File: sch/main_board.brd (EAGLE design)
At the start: 99.2 x 65.2 mm, 17 parts, among them IC1 MCP73831T-2ACI_OT

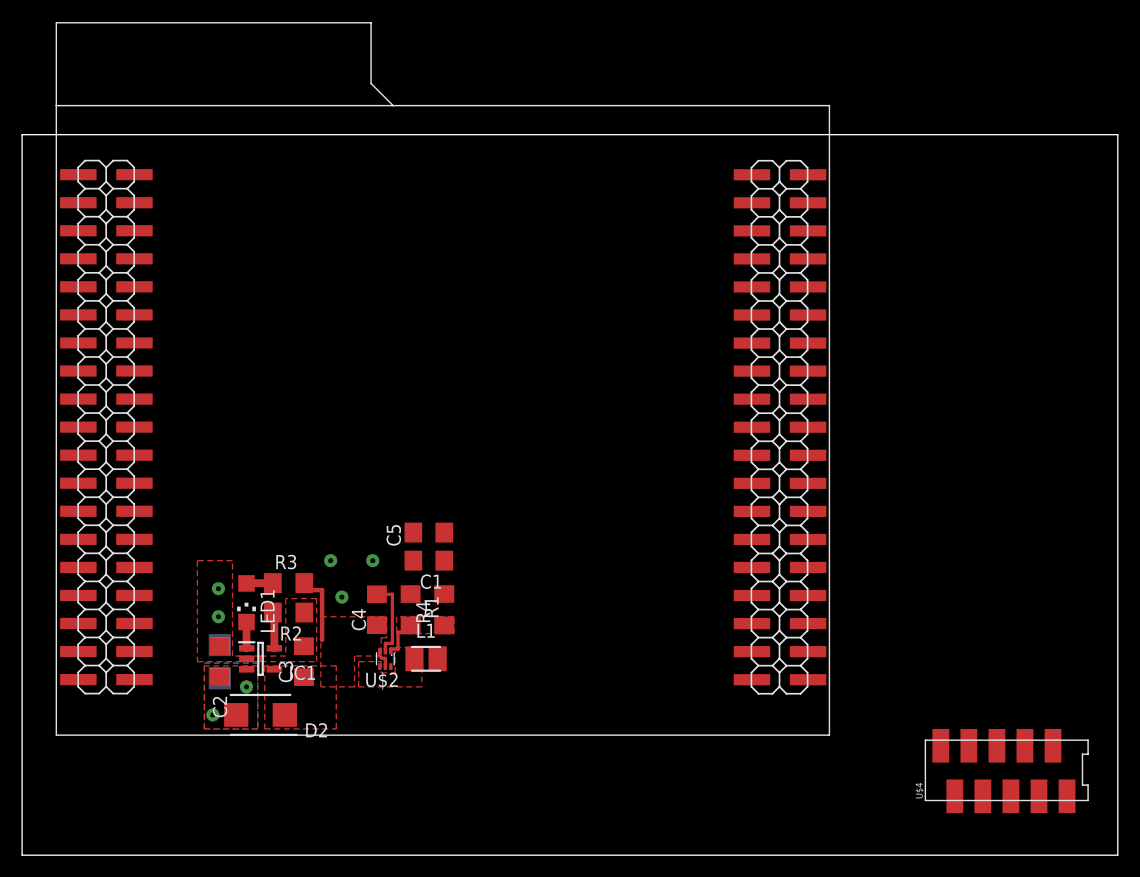
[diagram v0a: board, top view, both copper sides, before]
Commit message: Main board ver. 1.0
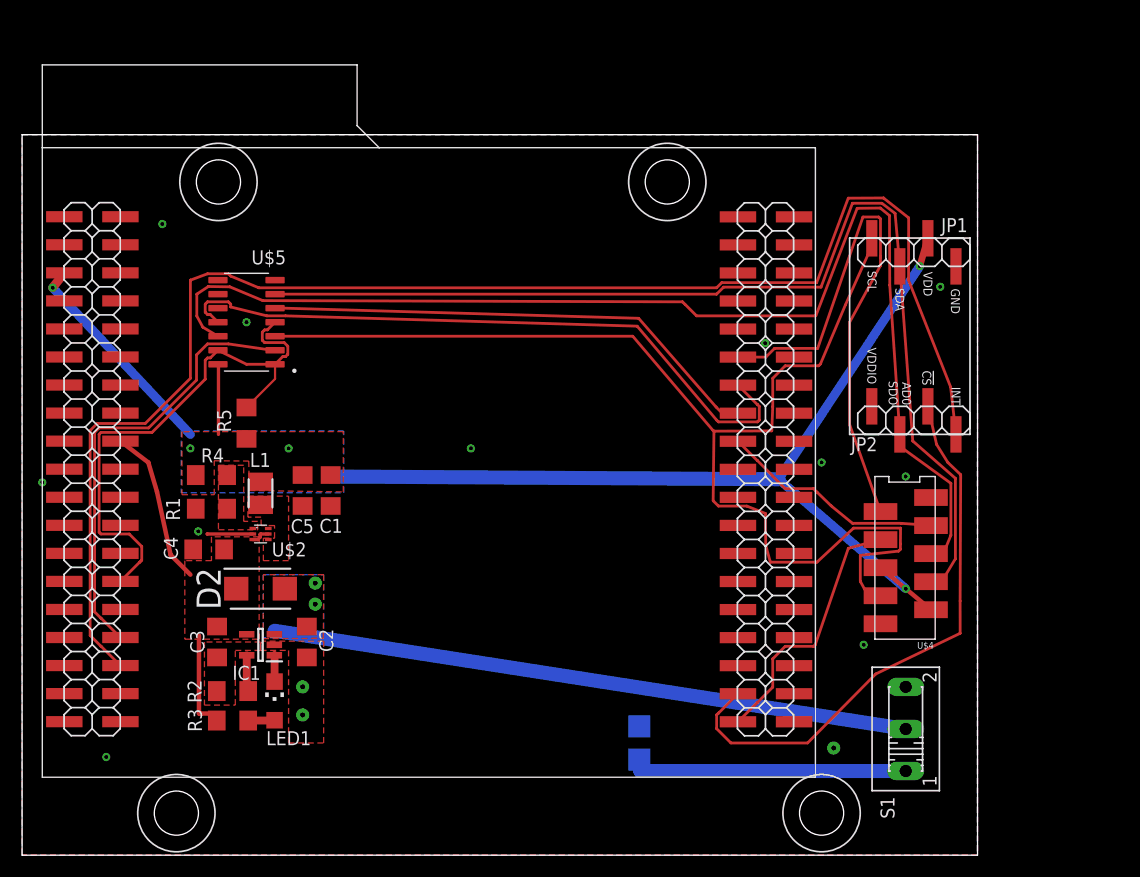
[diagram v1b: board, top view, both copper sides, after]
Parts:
- added JP1, JP2: (no value), pinhead-2:1X04SMD
- added R5: 10k, resistor:R1206
- added S1: (no value), switch:255SB
- added U$5: (no value), SamacSys_Parts:SOIC127P600X175-14N
- R4: value 316k -> 402k
- moved U$1 38.7 mm to (55.9, 10.2)
- moved R4 24.4 mm to (17.1, 34.4), turned to 180 degrees
- moved L1 21.2 mm to (21.6, 32.8), turned to 90 degrees
- moved U$4 21.0 mm to (80.0, 26.7), turned to 90 degrees
- moved R1 20.2 mm to (17.1, 31.4), turned to 0 degrees
- moved C4 16.2 mm to (16.9, 27.7), turned to 180 degrees
- moved U$2 16.0 mm to (21.6, 29.1), turned to 270 degrees
- moved R3 13.4 mm to (19.1, 12.2), turned to 180 degrees
- moved C5 12.0 mm to (25.4, 33.0), turned to 270 degrees
- moved D2 11.4 mm to (21.6, 24.1), turned to 0 degrees
- moved C1 10.9 mm to (27.9, 33.0), turned to 270 degrees
- moved LED1 9.25 mm to (22.9, 14.0), turned to 0 degrees
- moved R2 8.74 mm to (19.1, 14.9), turned to 0 degrees
- moved C3 8.07 mm to (17.7, 19.3), turned to 270 degrees
- moved C2 8.07 mm to (25.8, 19.3), turned to 270 degrees
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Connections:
- new net AD0/SDO: JP2.2, U$4.P$6, U$5.12
- new net BUFFER_EN: R5.1, U$3.28, U$5.1, U$5.13, U$5.4
- new net N$4: S1.1, U$1.P
- new net SCL/SCLK: JP1.1, U$4.P$3, U$5.3
- new net SDA/SDI: JP1.2, U$4.P$4, U$5.6
- net GND: now also JP1.4, U$5.10, U$5.7
- net MPU_INT: now also JP2.4; no longer U$4.P$5
- net SPI_CS_0: now also JP2.3
- net SPI_CS_1: now also U$4.P$7; no longer U$4.P$6
- net SPI_CS_2: now also U$4.P$8; no longer U$4.P$7
- net SPI_CS_3: now also U$4.P$9; no longer U$4.P$8
- net SPI_MISO: now also U$5.11; no longer U$4.P$9
- net SPI_MOSI: now also U$5.5; no longer U$4.P$4
- net SPI_SCK: now also U$5.2; no longer U$4.P$3
- net VCC: now also JP1.3, R5.2, U$4.P$5, U$5.14
- net V_BATT: now also S1.2; no longer U$1.P
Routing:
- net MPU_INT: track 0.00 -> 134.3 mm
- net VCC: track 0.00 -> 113.8 mm, vias 0 -> 5
- net SCL/SCLK: track 0.00 -> 110.1 mm
- net AD0/SDO: track 0.00 -> 109.4 mm
- net SDA/SDI: track 0.00 -> 98.3 mm
- net SPI_MISO: track 0.00 -> 61.0 mm
- net V_BATT: track 0.00 -> 57.8 mm
- net SPI_CS_0: track 0.00 -> 51.4 mm
- net BUFFER_EN: track 0.00 -> 49.7 mm
- net SPI_CS_3: track 0.00 -> 49.6 mm
- net SPI_MOSI: track 0.00 -> 46.0 mm
- net SPI_SCK: track 0.00 -> 40.6 mm
- net N$4: track 0.00 -> 25.1 mm, vias 1 -> 0
- net SPI_CS_1: track 0.00 -> 23.6 mm
- net SPI_CS_2: track 0.00 -> 20.8 mm
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- added copper zone on layer 16, net GND
- added copper zone on layer 1, net VCC
- added copper zone on layer 16, net VCC
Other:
- board size 99.2 x 65.2 mm -> 86.5 x 65.2 mm
- board text added: "!CS"
- board text added: "AD0 SDO"
- board text added: "BATT"
- board text added: "GND"
- board text added: "INT"
- board text added: "Praca Magisterska AGH, Elektronika i Telekomunikacja, Systemy Wbudowane Autor: Damian Świerk 2019"
- board text added: "SCL"
- board text added: "SDA"
- board text added: "VDD"
- board text added: "VDDIO"
